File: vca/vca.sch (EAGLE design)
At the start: 36 parts, among them IC1 OPA4130U, IC2 OPA134D, IC3 OPA2134D, X1 2516-

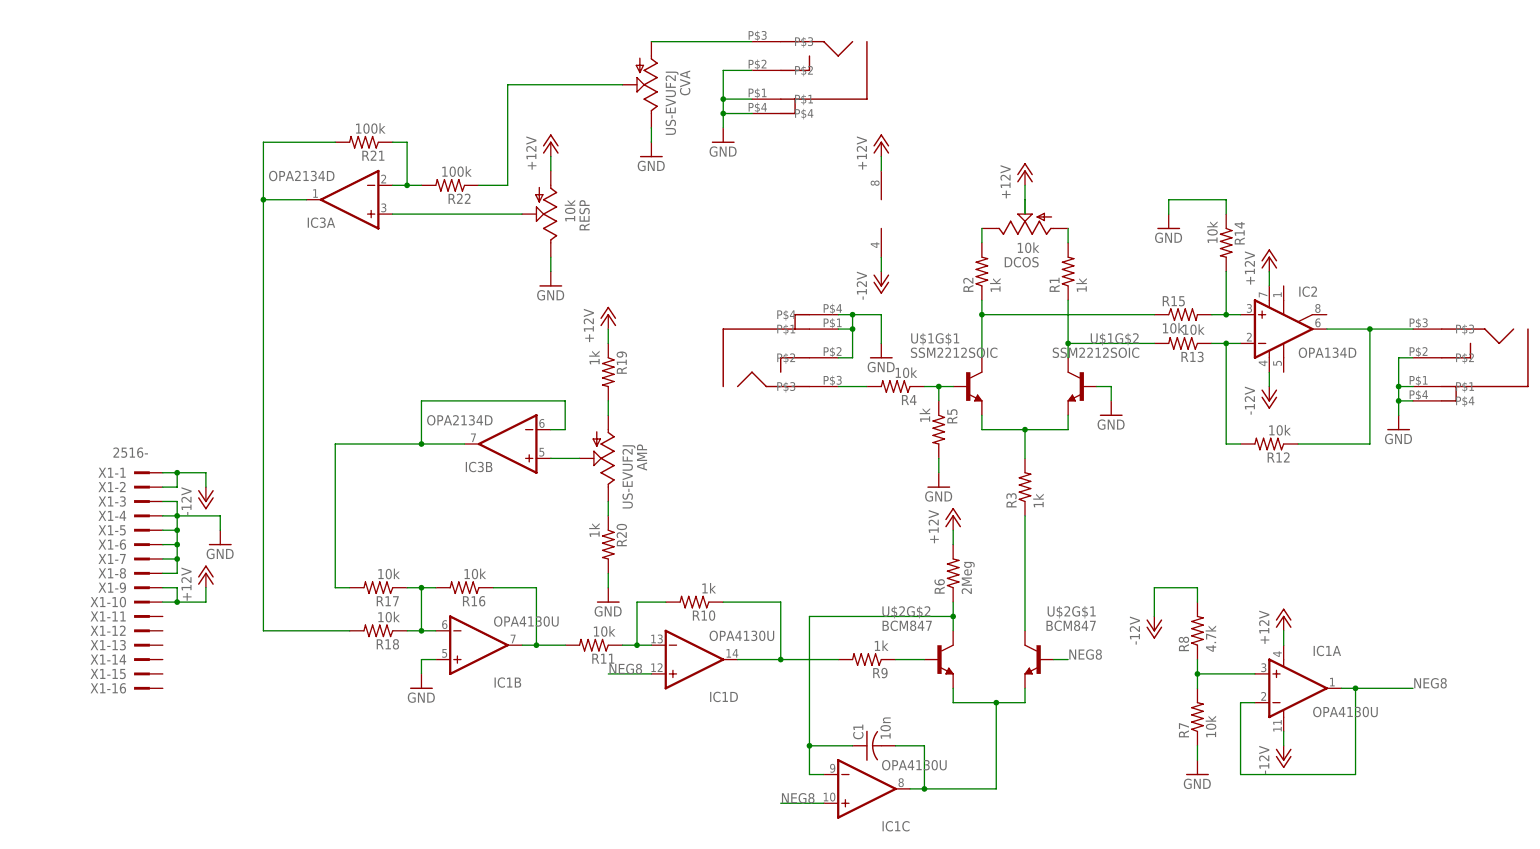
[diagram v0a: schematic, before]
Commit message: almost got the vca pcb done
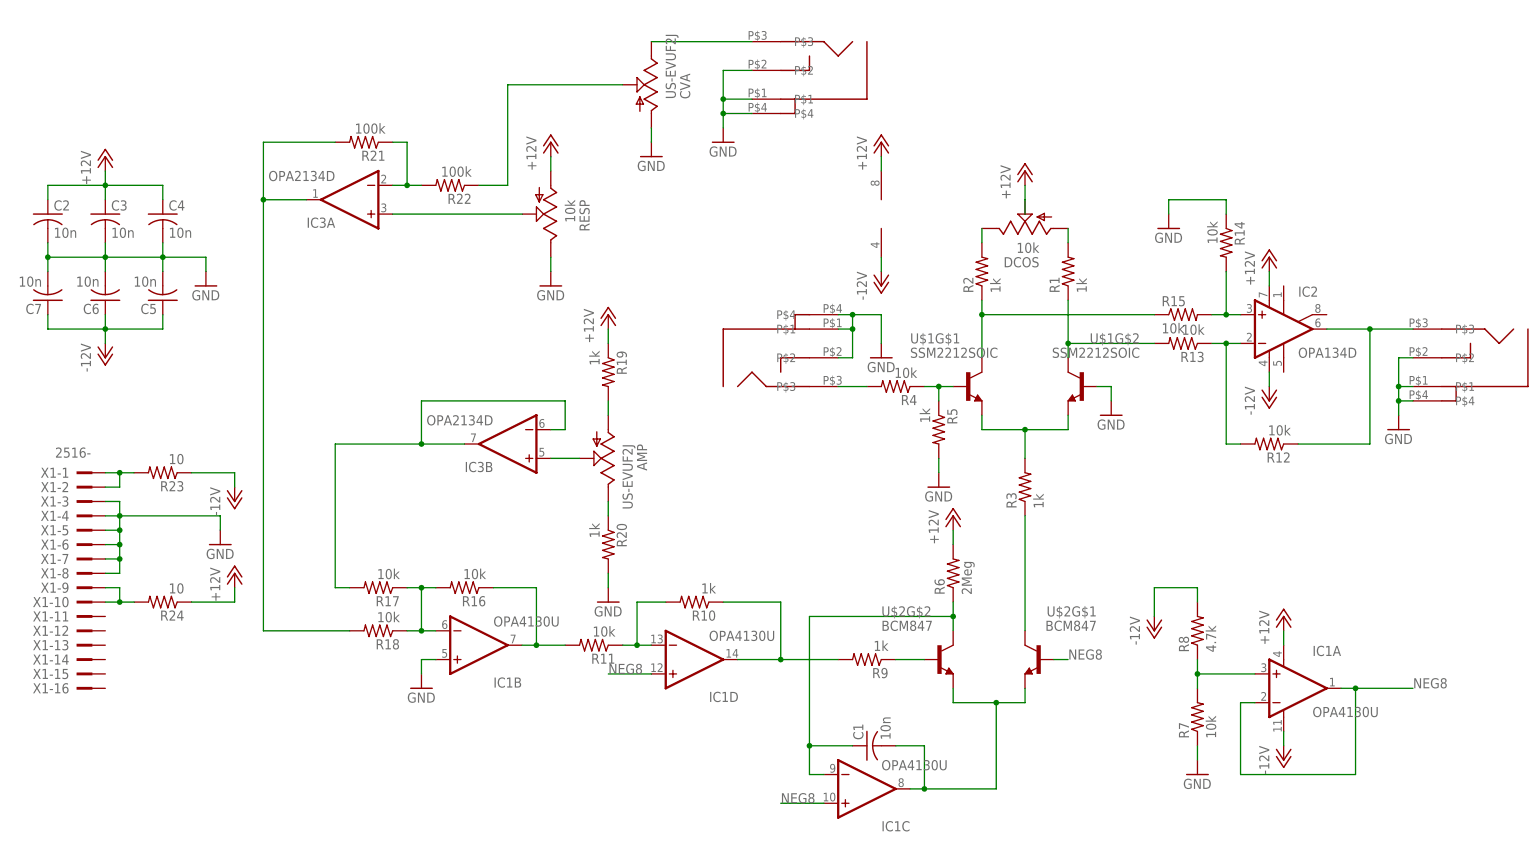
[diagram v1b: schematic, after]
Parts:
- added C2, C3, C4, C5, C6, C7: 10n, dan:C-USC0603
- added R23, R24: 10, dan:R-US_R0603
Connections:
- new net N$30: R23.2, X1-1.KL, X1-2.KL
- new net N$34: R24.2, X1-10.KL, X1-9.KL
- net +12V: now also C2.1, C3.1, C4.1, R24.1; no longer X1-10.KL, X1-9.KL
- net -12V: now also C5.1, C6.1, C7.1, R23.1; no longer X1-1.KL, X1-2.KL
- net GND: now also C2.2, C3.2, C4.2, C5.2, C6.2, C7.2, CVA.A; no longer CVA.E
- net N$26: now also CVA.E; no longer CVA.A
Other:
- moved on the sheet: CVA, X1-1, X1-10, X1-11, X1-12, X1-13, X1-14, X1-15, X1-16, X1-2, X1-3, X1-4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
